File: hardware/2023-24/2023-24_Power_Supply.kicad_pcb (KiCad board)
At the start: 2 copper layers, 325 x 235 mm, 272 parts, among them J10 Screw_Terminal_01x01, J11 TBL007A-508-06GY, J12 Conn_01x02, J13 Screw_Terminal_01x06, J14 Screw_Terminal_01x06, J15 Screw_Terminal_01x06, J16 Conn_01x05_Pin, J17 Conn_01x05_Pin, J18 Conn_01x05_Pin, J20 Conn_01x05_Pin, J21 Conn_01x05_Pin, J22 Conn_01x05_Pin, J23 Conn_01x05_Pin, J24 Conn_01x05_Pin, J4 Screw_Terminal_01x01, J5 Screw_Terminal_01x01, J6 Screw_Terminal_01x01, J7 Screw_Terminal_01x01, J8 TBL007A-508-06GY, J9 Screw_Terminal_01x01, K1 G9KB-1A-E DC12, Q17 PNP, Q18 NMOS, Q26 PNP, Q27 NMOS, Q28 NMOS, Q29 NMOS, Q30 NMOS, Q8 PNP, Q9 NMOS, U10 ADS1015IDGS, U12 LM5066, U14 LM5066, U16 LM5066, U5 LM5066, U6 LM5066, U7 LM5066, U9 ADS1015IDGS

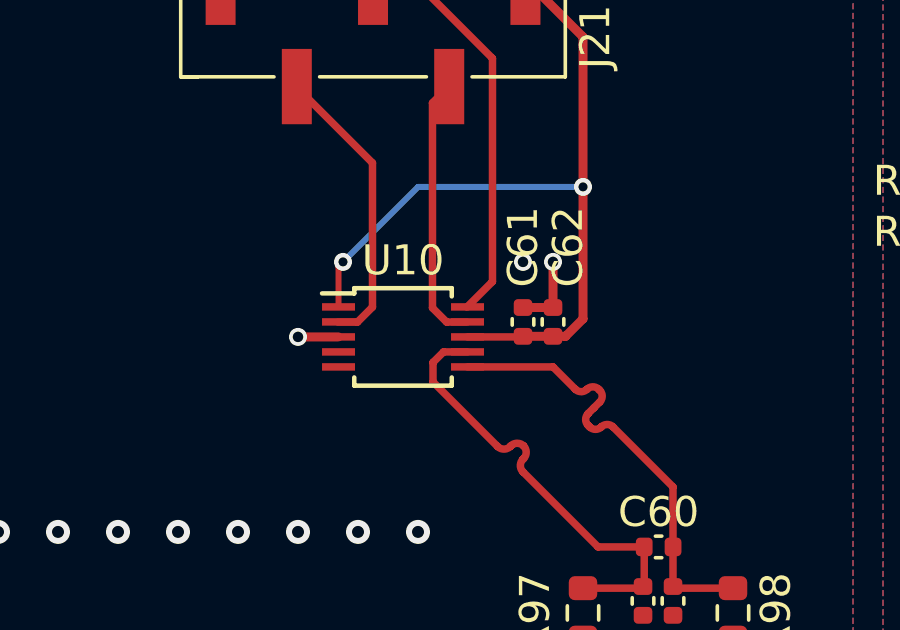
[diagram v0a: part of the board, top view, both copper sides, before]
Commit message: Pushing for pre-production review
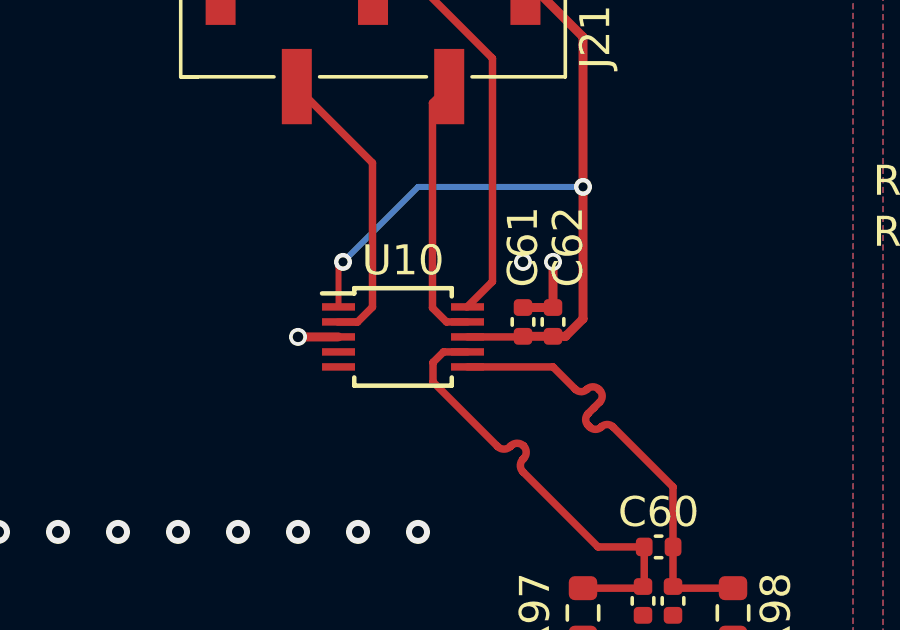
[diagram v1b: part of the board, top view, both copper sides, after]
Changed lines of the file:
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@@
       (plot_on_all_layers_selection 0x0000000_00000000)
       (disableapertmacros false)
-      (usegerberextensions false)
+      (usegerberextensions true)
       (usegerberattributes true)
       (usegerberadvancedattributes true)
-      (creategerberjobfile true)
+      (creategerberjobfile false)
       (dashed_line_dash_ratio 12.000000)
       (dashed_line_gap_ratio 3.000000)
@@
       (plotinvisibletext false)
       (sketchpadsonfab false)
-      (subtractmaskfromsilk false)
+      (subtractmaskfromsilk true)
       (outputformat 1)
       (mirror false)
-      (drillshape 1)
+      (drillshape 0)
       (scaleselection 1)
-      (outputdirectory "")
+      (outputdirectory "gerbers/")
     )
   )
@@
   (segment (start 254.28 212.908909) (end 255.6 211.588909) (width 0.35) (layer "F.Cu") (net 107))
   (segment (start 273.6 211.588909) (end 276.011091 214) (width 0.35) (layer "F.Cu") (net 107))
-  (segment (start 324.4535 245.505) (end 323.9825 245.034) (width 0.25) (layer "F.Cu") (net 108))
   (segment (start 237.15 245.5) (end 236.471 245.5) (width 0.25) (layer "F.Cu") (net 108))
+  (segment (start 325.15 245.5) (end 324.4485 245.5) (width 0.25) (layer "F.Cu") (net 108))
+  (segment (start 324.4485 245.5) (end 323.9825 245.034) (width 0.25) (layer "F.Cu") (net 108))
   (segment (start 323.9825 245.034) (end 323.9825 238.2) (width 0.25) (layer "F.Cu") (net 108))
   (segment (start 236 238.195) (end 236.54 237.655) (width 0.25) (layer "F.Cu") (net 108))
   (segment (start 236.471 245.5) (end 236 245.029) (width 0.25) (layer "F.Cu") (net 108))
-  (segment (start 325.1325 245.505) (end 324.4535 245.505) (width 0.25) (layer "F.Cu") (net 108))
   (segment (start 236 245.029) (end 236 238.195) (width 0.25) (layer "F.Cu") (net 108))
   (segment (start 323.9825 238.2) (end 324.5225 237.66) (width 0.25) (layer "F.Cu") (net 108))
